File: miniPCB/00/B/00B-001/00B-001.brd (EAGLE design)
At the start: 27 parts, among them U1 324

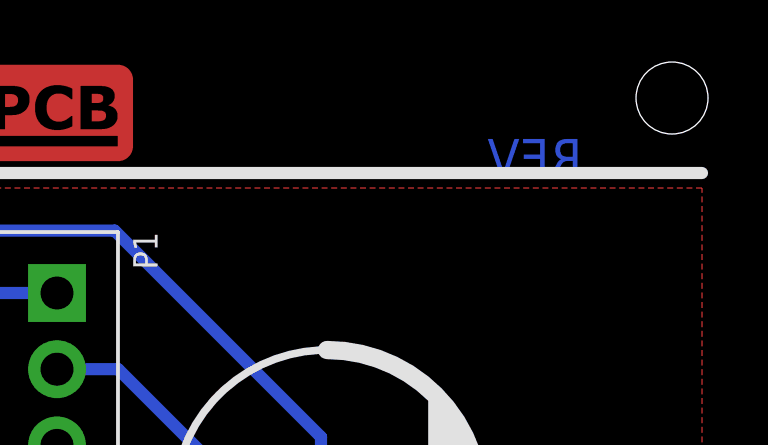
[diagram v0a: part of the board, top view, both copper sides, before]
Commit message: NM.23OCT2023
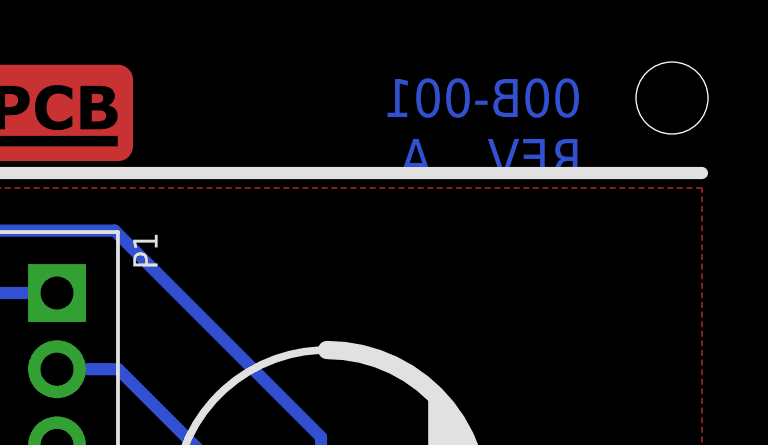
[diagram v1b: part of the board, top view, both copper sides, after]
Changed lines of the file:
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@@
 <?xml version="1.0" encoding="utf-8"?>
 <!DOCTYPE eagle SYSTEM "eagle.dtd">
-<eagle version="6.3">
+<eagle version="9.6.2">
 <drawing>
 <settings>
 <setting alwaysvectorfont="no"/>
+<setting keepoldvectorfont="yes"/>
 <setting verticaltext="up"/>
 </settings>
@@
 <layer number="59" name="tCarbon" color="7" fill="1" visible="no" active="no"/>
 <layer number="60" name="bCarbon" color="7" fill="1" visible="no" active="no"/>
-<layer number="88" name="SimResults" color="9" fill="1" visible="yes" active="yes"/>
-<layer number="89" name="SimProbes" color="9" fill="1" visible="yes" active="yes"/>
-<layer number="90" name="Modules" color="7" fill="1" visible="yes" active="yes"/>
+<layer number="88" name="SimResults" color="9" fill="1" visible="no" active="no"/>
+<layer number="89" name="SimProbes" color="9" fill="1" visible="no" active="no"/>
+<layer number="90" name="Modules" color="7" fill="1" visible="no" active="no"/>
 <layer number="91" name="Nets" color="2" fill="1" visible="no" active="no"/>
 <layer number="92" name="Busses" color="1" fill="1" visible="no" active="no"/>
@@
 <param name="dpMaxLengthDifference" value="10mm"/>
 <param name="dpGapFactor" value="2.5"/>
-<param name="checkGrid" value="0"/>
 <param name="checkAngle" value="0"/>
 <param name="checkFont" value="1"/>
 <param name="checkRestrict" value="1"/>
+<param name="checkStop" value="0"/>
+<param name="checkValues" value="0"/>
+<param name="checkNames" value="1"/>
+<param name="checkWireStubs" value="1"/>
+<param name="checkPolygonWidth" value="0"/>
 <param name="useDiameter" value="13"/>
 <param name="maxErrors" value="50"/>
@@
 <pass name="Default">
 <param name="RoutingGrid" value="50mil"/>
+<param name="AutoGrid" value="1"/>
+<param name="Efforts" value="0"/>
+<param name="TopRouterVariant" value="1"/>
 <param name="tpViaShape" value="round"/>
 <param name="PrefDir.1" value="|"/>
@@
 </autorouter>
 <elements>
-<element name="U1" library="minipcb" package="DIL14" value="324" x="32.5" y="18.5"/>
+<element name="U1" library="minipcb" package="DIL14" value="324" x="32.5" y="18.5" smashed="yes">
+<attribute name="NAME" x="23.229" y="15.452" size="0.8128" layer="25" font="vector" ratio="12" rot="R90"/>
+<attribute name="VALUE" x="25.769" y="17.865" size="1.27" layer="27" ratio="10"/>
+</element>
 <element name="C1" library="minipcb" package="C050-024X044" value="1u" x="29.5" y="10.5" smashed="yes" rot="R180">
 <attribute name="NAME" x="27.5" y="12" size="0.8128" layer="25" font="vector" ratio="13"/>
 </element>
-<element name="P1" library="minipcb" package="TRIM_0100" value="" x="27.5" y="41.5" rot="R270"/>
-<element name="R5" library="minipcb" package="0207/10" value="" x="22.5" y="38.5" rot="R90"/>
-<element name="R6" library="minipcb" package="0207/10" value="" x="18.5" y="38.5" rot="R90"/>
-<element name="C2" library="minipcb" package="C5MM" value="" x="36.5" y="34.5"/>
+<element name="P1" library="minipcb" package="TRIM_0100" value="" x="27.5" y="41.5" smashed="yes" rot="R270">
+<attribute name="NAME" x="30.04" y="43.532" size="0.8128" layer="25" font="vector" ratio="12" rot="R270"/>
+</element>
+<element name="R5" library="minipcb" package="0207/10" value="" x="22.5" y="38.5" smashed="yes" rot="R90">
+<attribute name="NAME" x="20.976" y="35.452" size="0.8128" layer="25" font="vector" ratio="12" rot="R90"/>
+<attribute name="VALUE" x="22.5" y="38.5" size="0.8128" layer="27" font="vector" ratio="12" rot="R90" align="center"/>
+</element>
+<element name="R6" library="minipcb" package="0207/10" value="" x="18.5" y="38.5" smashed="yes" rot="R90">
+<attribute name="NAME" x="16.976" y="35.452" size="0.8128" layer="25" font="vector" ratio="12" rot="R90"/>
+<attribute name="VALUE" x="18.5" y="38.5" size="0.8128" layer="27" font="vector" ratio="12" rot="R90" align="center"/>
+</element>
+<element name="C2" library="minipcb" package="C5MM" value="" x="36.5" y="34.5" smashed="yes">
+<attribute name="NAME" x="31" y="33" size="0.8128" layer="25" font="vector" ratio="12" rot="R180"/>
+</element>
 <element name="C3" library="minipcb" package="C050-024X044" value="" x="28.5" y="29.5" smashed="yes" rot="R90">
 <attribute name="NAME" x="27" y="27.5" size="0.8128" layer="25" font="vector" ratio="13" rot="R90"/>
@@
 <attribute name="VALUE" x="8.5" y="37.5" size="0.8128" layer="27" font="vector" ratio="12" rot="R180" align="center"/>
 </element>
-<element name="TP4" library="minipcb" package="PINS_1_TESTPOINT_KE5000_NOTEXT" value="" x="24.5" y="26.5" rot="R90"/>
+<element name="TP4" library="minipcb" package="PINS_1_TESTPOINT_KE5000_NOTEXT" value="" x="24.5" y="26.5" smashed="yes" rot="R90">
+<attribute name="NAME" x="23.23" y="26.5" size="0.8128" layer="25" font="vector" ratio="12" rot="R90" align="bottom-center"/>
+</element>
 <element name="R3" library="minipcb" package="0207/10" value="" x="28.5" y="6.5" smashed="yes">
 <attribute name="NAME" x="25.452" y="8.024" size="0.8128" layer="25" font="vector" ratio="12"/>
@@
 <attribute name="VALUE" x="8.5" y="20.5" size="0.8128" layer="27" font="vector" ratio="12" align="center"/>
 </element>
-<element name="C4" library="minipcb" package="C050-024X044" value="" x="17.5" y="18.5" rot="R90"/>
+<element name="C4" library="minipcb" package="C050-024X044" value="" x="17.5" y="18.5" smashed="yes" rot="R90">
+<attribute name="NAME" x="16" y="16.5" size="0.8128" layer="25" font="vector" ratio="13" rot="R90"/>
+<attribute name="VALUE" x="19" y="20.5" size="0.8128" layer="27" font="vector" ratio="13" rot="R270"/>
+</element>
 <element name="R9" library="minipcb" package="0207/10" value="" x="8.5" y="24.5" smashed="yes" rot="R180">
 <attribute name="NAME" x="5.452" y="26.024" size="0.8128" layer="25" font="vector" ratio="12"/>
@@
 <attribute name="VALUE" x="6.5" y="30.5" size="0.8128" layer="27" font="vector" ratio="13"/>
 </element>
-<element name="TP5" library="minipcb" package="PINS_1_TESTPOINT_KE5000_NOTEXT" value="" x="20.5" y="17" rot="R180"/>
-<element name="TP6" library="minipcb" package="PINS_1_TESTPOINT_KE5000_NOTEXT" value="" x="20.5" y="20"/>
-<element name="TP7" library="minipcb" package="PINS_1_TESTPOINT_KE5000_NOTEXT" value="" x="17.5" y="24.5" rot="R270"/>
-<element name="TP8" library="minipcb" package="PINS_1_TESTPOINT_KE5000_NOTEXT" value="" x="17.5" y="27.5" rot="R270"/>
-<element name="TP3" library="minipcb" package="PINS_1_TESTPOINT_KE5000_NOTEXT" value="" x="2.5" y="8" rot="R270"/>
-<element name="TP1" library="minipcb" package="PINS_1_TESTPOINT_KE5000_NOTEXT" value="" x="17.5" y="3.5" rot="R90"/>
-<element name="J7-" library="minipcb" package="MINIPCB_5P_50X50MM" value="" x="0" y="0">
-<attribute name="REVISION" value="A" x="0" y="0" size="1.778" layer="27" display="off"/>
-<attribute name="PART_NUMBER" value="00B-001" x="0" y="0" size="1.778" layer="27" display="off"/>
-</element>
-<element name="TP2" library="minipcb" package="PINS_1_TESTPOINT_KE5000_NOTEXT" value="" x="17.5" y="7" rot="R90"/>
+<element name="TP5" library="minipcb" package="PINS_1_TESTPOINT_KE5000_NOTEXT" value="" x="20.5" y="17" smashed="yes" rot="R180">
+<attribute name="NAME" x="20.5" y="15.73" size="0.8128" layer="25" font="vector" ratio="12" rot="R180" align="bottom-center"/>
+</element>
+<element name="TP6" library="minipcb" package="PINS_1_TESTPOINT_KE5000_NOTEXT" value="" x="20.5" y="20" smashed="yes">
+<attribute name="NAME" x="20.5" y="21.27" size="0.8128" layer="25" font="vector" ratio="12" align="bottom-center"/>
+</element>
+<element name="TP7" library="minipcb" package="PINS_1_TESTPOINT_KE5000_NOTEXT" value="" x="17.5" y="24.5" smashed="yes" rot="R270">
+<attribute name="NAME" x="18.77" y="24.5" size="0.8128" layer="25" font="vector" ratio="12" rot="R270" align="bottom-center"/>
+</element>
+<element name="TP8" library="minipcb" package="PINS_1_TESTPOINT_KE5000_NOTEXT" value="" x="17.5" y="27.5" smashed="yes" rot="R270">
+<attribute name="NAME" x="18.77" y="27.5" size="0.8128" layer="25" font="vector" ratio="12" rot="R270" align="bottom-center"/>
+</element>
+<element name="TP3" library="minipcb" package="PINS_1_TESTPOINT_KE5000_NOTEXT" value="" x="2.5" y="8" smashed="yes" rot="R270">
+<attribute name="NAME" x="3.77" y="8" size="0.8128" layer="25" font="vector" ratio="12" rot="R270" align="bottom-center"/>
+</element>
+<element name="TP1" library="minipcb" package="PINS_1_TESTPOINT_KE5000_NOTEXT" value="" x="17.5" y="3.5" smashed="yes" rot="R90">
+<attribute name="NAME" x="16.23" y="3.5" size="0.8128" layer="25" font="vector" ratio="12" rot="R90" align="bottom-center"/>
+</element>
+<element name="J7-" library="minipcb" package="MINIPCB_5P_50X50MM" value="" x="0" y="0" smashed="yes">
+<attribute name="PART_NUMBER" value="00B-001" x="45" y="48" size="1.27" layer="16" font="vector" ratio="13" rot="MR180" align="center-right"/>
+<attribute name="REVISION" value="A" x="40" y="46" size="1.27" layer="16" font="vector" ratio="13" rot="MR180" align="center-right"/>
+</element>
+<element name="TP2" library="minipcb" package="PINS_1_TESTPOINT_KE5000_NOTEXT" value="" x="17.5" y="7" smashed="yes" rot="R90">
+<attribute name="NAME" x="16.23" y="7" size="0.8128" layer="25" font="vector" ratio="12" rot="R90" align="bottom-center"/>
+</element>
 </elements>
 <signals>
@@
 </signal>
 </signals>
+<mfgpreviewcolors>
+<mfgpreviewcolor name="soldermaskcolor" color="0xC8008000"/>
+<mfgpreviewcolor name="silkscreencolor" color="0xFFFEFEFE"/>
+<mfgpreviewcolor name="backgroundcolor" color="0xFF282828"/>
+<mfgpreviewcolor name="coppercolor" color="0xFFFFBF00"/>
+<mfgpreviewcolor name="substratecolor" color="0xFF786E46"/>
+</mfgpreviewcolors>
 </board>
 </drawing>
